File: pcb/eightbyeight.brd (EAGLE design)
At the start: 60 x 60 mm, 163 parts, among them CON1 USB_MICROSMT+THRUHULE, Q1 16MHz, SW1 SWITCH_SPDT, SW2 BRIGHTNESS, U1 MK20DN64VFM5, U10 FDG6316P, U11 FDG6316P, U12 FDG6316P, U2 ICN2026, U3 74138, U4 ICN2026, U5 MIC5219 3.3V, U6 ESP_WROOM_02, U8 MMA8653FC, U9 FDG6316P

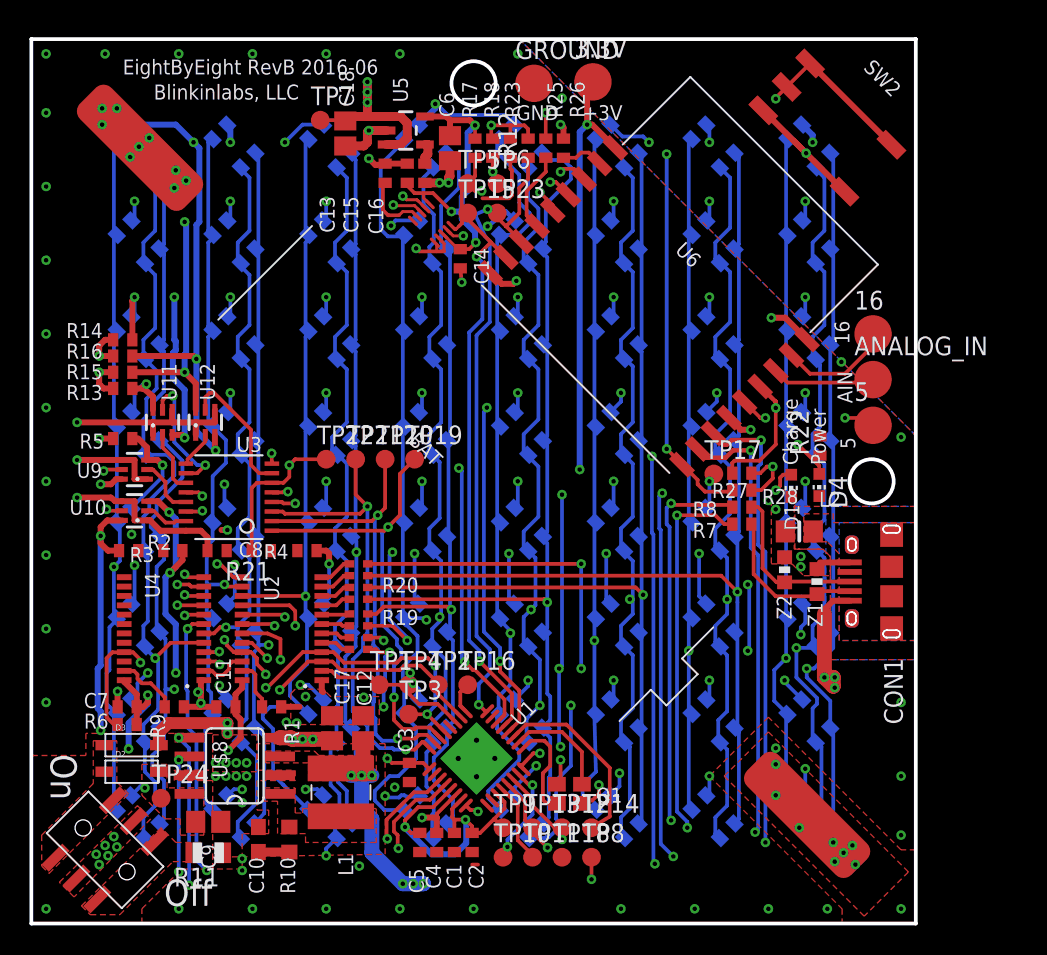
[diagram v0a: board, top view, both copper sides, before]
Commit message: Closer to RevD
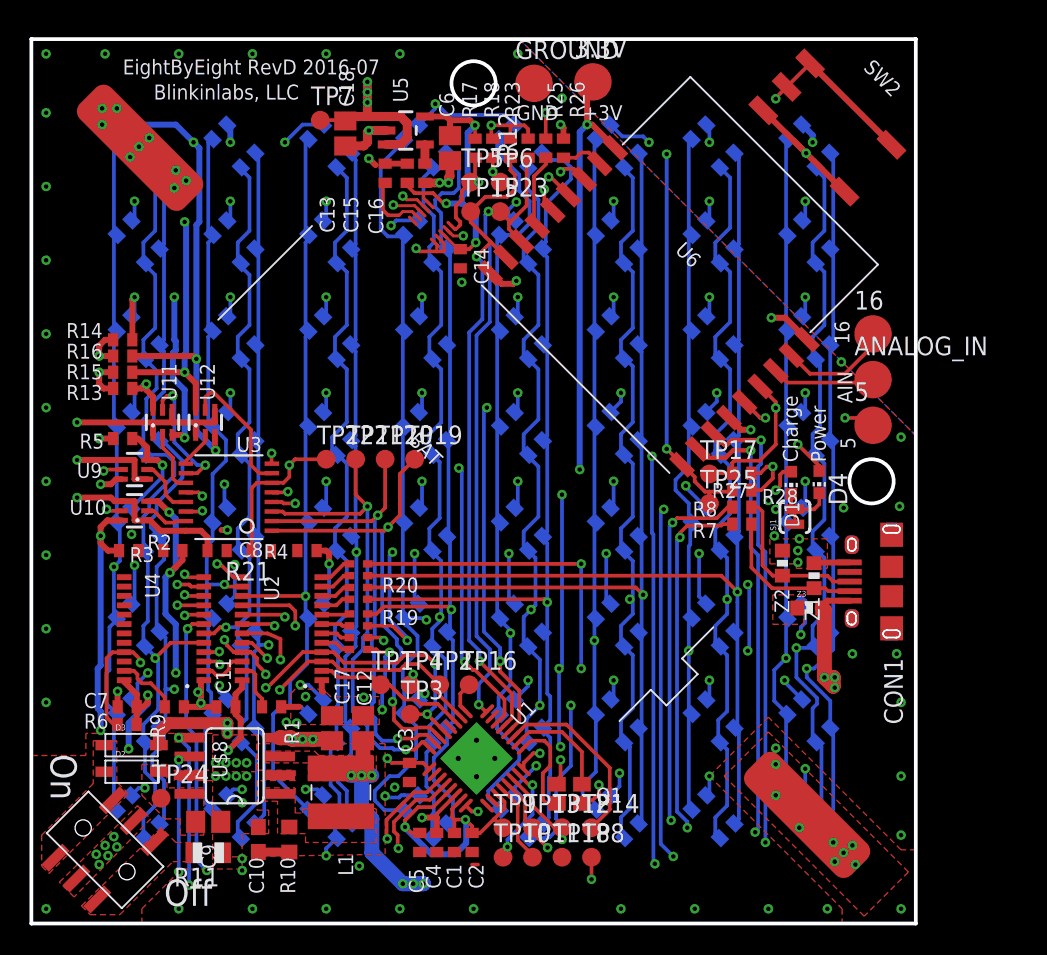
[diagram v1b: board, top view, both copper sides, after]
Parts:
- removed L2: 130ohm @100MHz, blinkinlabs:0805
- removed R22: 100, adafruit:R0402
- added SJ1: SOLDERJUMPERTRACE, SparkFun-Passives:SJ_2S-TRACE
- added TP25: PTR1B1,27, testpad:B1,27
- added Z3: PGB1010603, PaxInstrument-T400:SPARKFUN-RESISTORS_0603-RES
- moved Z2 0.47 mm to (51.0, 24.4)
- moved Z1 0.45 mm to (53.1, 23.6)
- moved TP17 0.30 mm to (46.0, 30.5)
- moved TP15 0.22 mm to (29.8, 48.3)
- moved TP23 0.22 mm to (31.8, 48.3)
- moved TP5 0.22 mm to (29.8, 50.3)
- moved TP6 0.22 mm to (31.8, 50.3)
- moved D1 0.20 mm to (51.5, 29.9)
- moved D4 0.20 mm to (53.5, 29.9)
- moved TP1 0.10 mm to (23.7, 16.2)
- moved TP16 0.10 mm to (29.7, 16.2)
- moved TP2 0.10 mm to (27.7, 16.2)
- moved TP3 0.10 mm to (25.7, 14.2)
- moved TP4 0.10 mm to (25.7, 16.2)
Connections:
- removed net BUTTON1: R28.1, SW2.1, SW2.2, U6.IO4
- removed net SHIELD: CON1.PAD$1, CON1.PAD$10, CON1.PAD$2, CON1.PAD$3, CON1.PAD$4, CON1.PAD$5, CON1.PAD$6, CON1.PAD$7, CON1.PAD$8, CON1.PAD$9, L2.1
- new net BUTTON: R28.1, SW2.1, SW2.2, TP25.TP, U6.IO4
- net GND: now also CON1.PAD$1, CON1.PAD$10, CON1.PAD$2, CON1.PAD$3, CON1.PAD$4, CON1.PAD$5, CON1.PAD$6, CON1.PAD$7, CON1.PAD$8, CON1.PAD$9, SJ1.1, Z3.1; no longer L2.2, R22.1
- net N$1: now also SJ1.2; no longer R22.2
- net USB_5V: now also Z3.2
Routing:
- net BUTTON: track 0.00 -> 45.3 mm, vias 0 -> 3
- net BUTTON1: track 44.5 -> 0.00 mm, vias 3 -> 0
- net GND: track 90.8 -> 74.9 mm, vias 88 -> 94
- net N$1: track 0.00 -> 3.69 mm
- net BCOL2: track 56.4 -> 54.6 mm
- net ESP_RESET: track 51.6 -> 53.1 mm
- net USB_D-: track 52.3 -> 51.0 mm
- net USB_D+: track 52.2 -> 51.0 mm
- net 1ROW1: track 74.3 -> 73.1 mm
- net ESP_GPIO0: track 44.0 -> 45.3 mm
- net ARM_RX1: track 45.0 -> 43.9 mm
- net N$9: track 11.2 -> 10.3 mm
- net RCOL3: track 54.5 -> 55.3 mm
- net ACC_INT1: track 14.2 -> 15.0 mm
- net BCOL6: track 79.0 -> 79.7 mm
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- removed copper zone on layer 1, net SHIELD
- removed copper zone on layer 16, net SHIELD
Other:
- board text added: "EightByEight RevD 2016-07"
- board text removed: "EightByEight RevB 2016-06"
